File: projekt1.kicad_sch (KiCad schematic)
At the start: 19 parts, among them U1 M5STAMP-S3, U3 SCD42, U4 RV-3028-C7

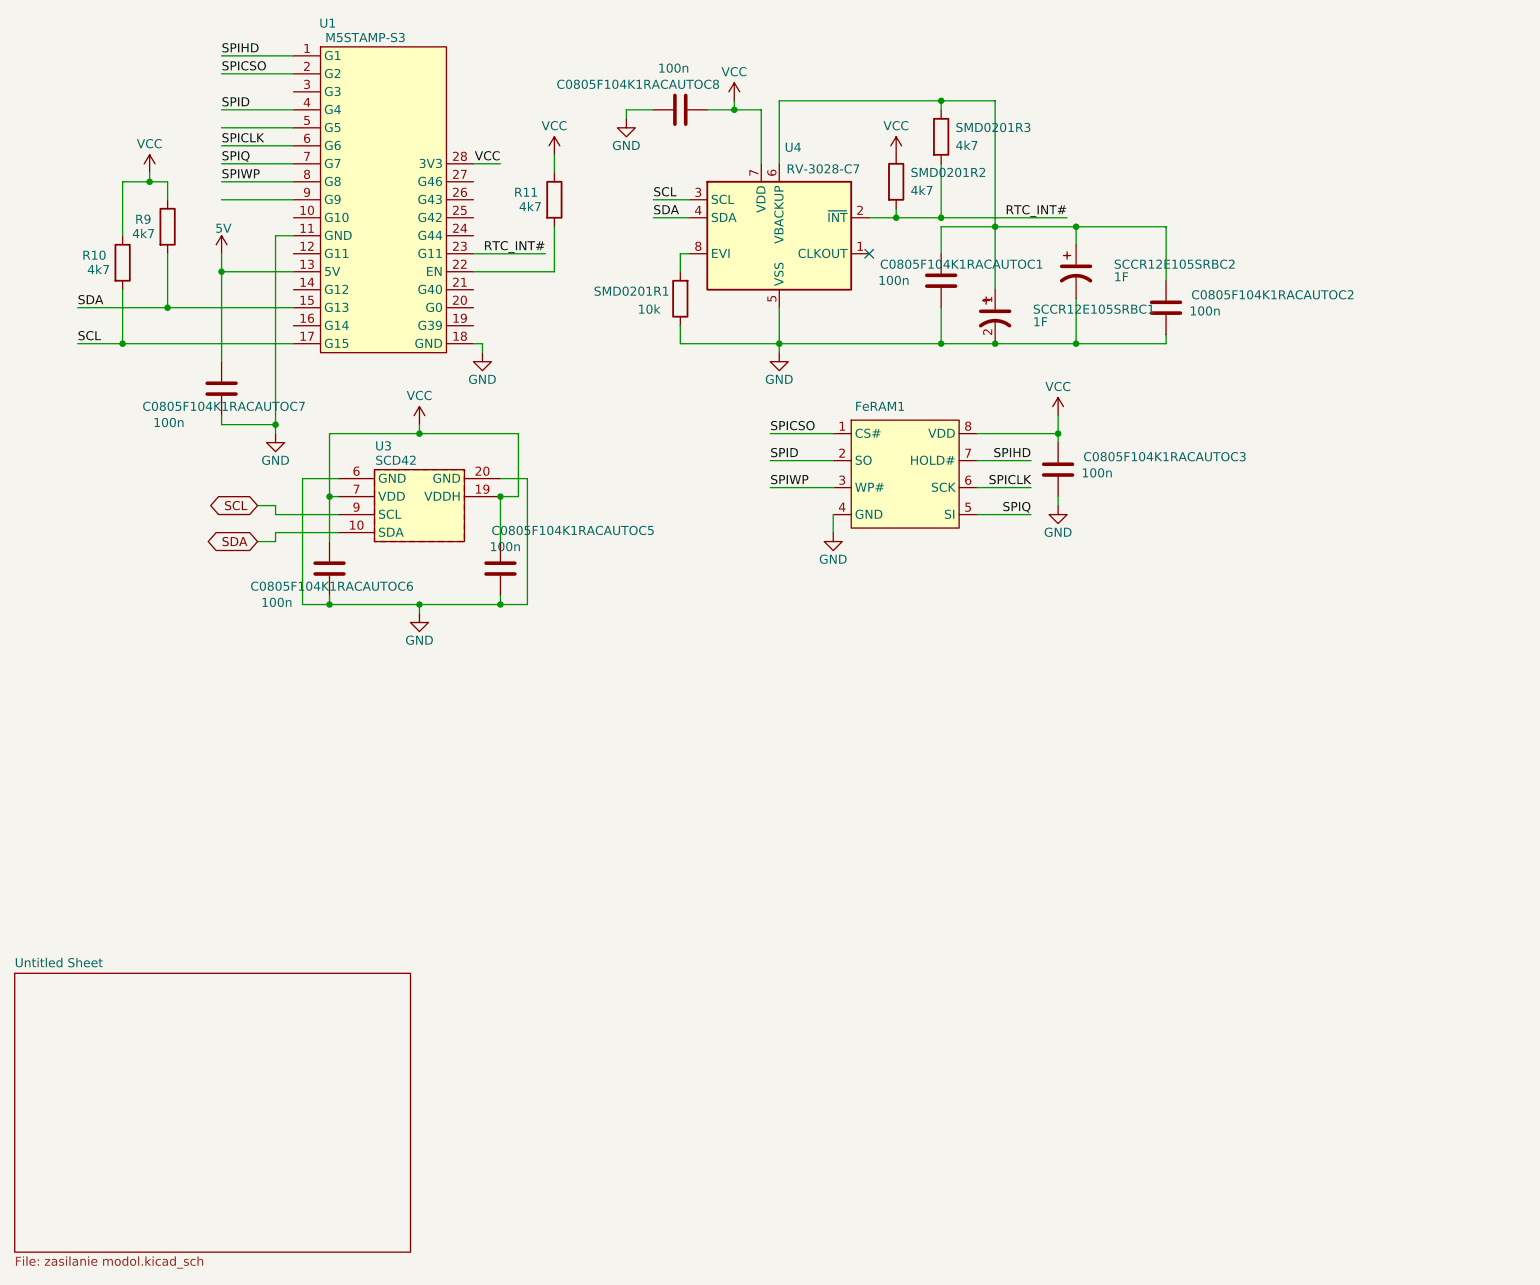
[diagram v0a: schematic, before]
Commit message: aaaaaaaaaaaaaaaaaaaaaaaaaaaaaaa
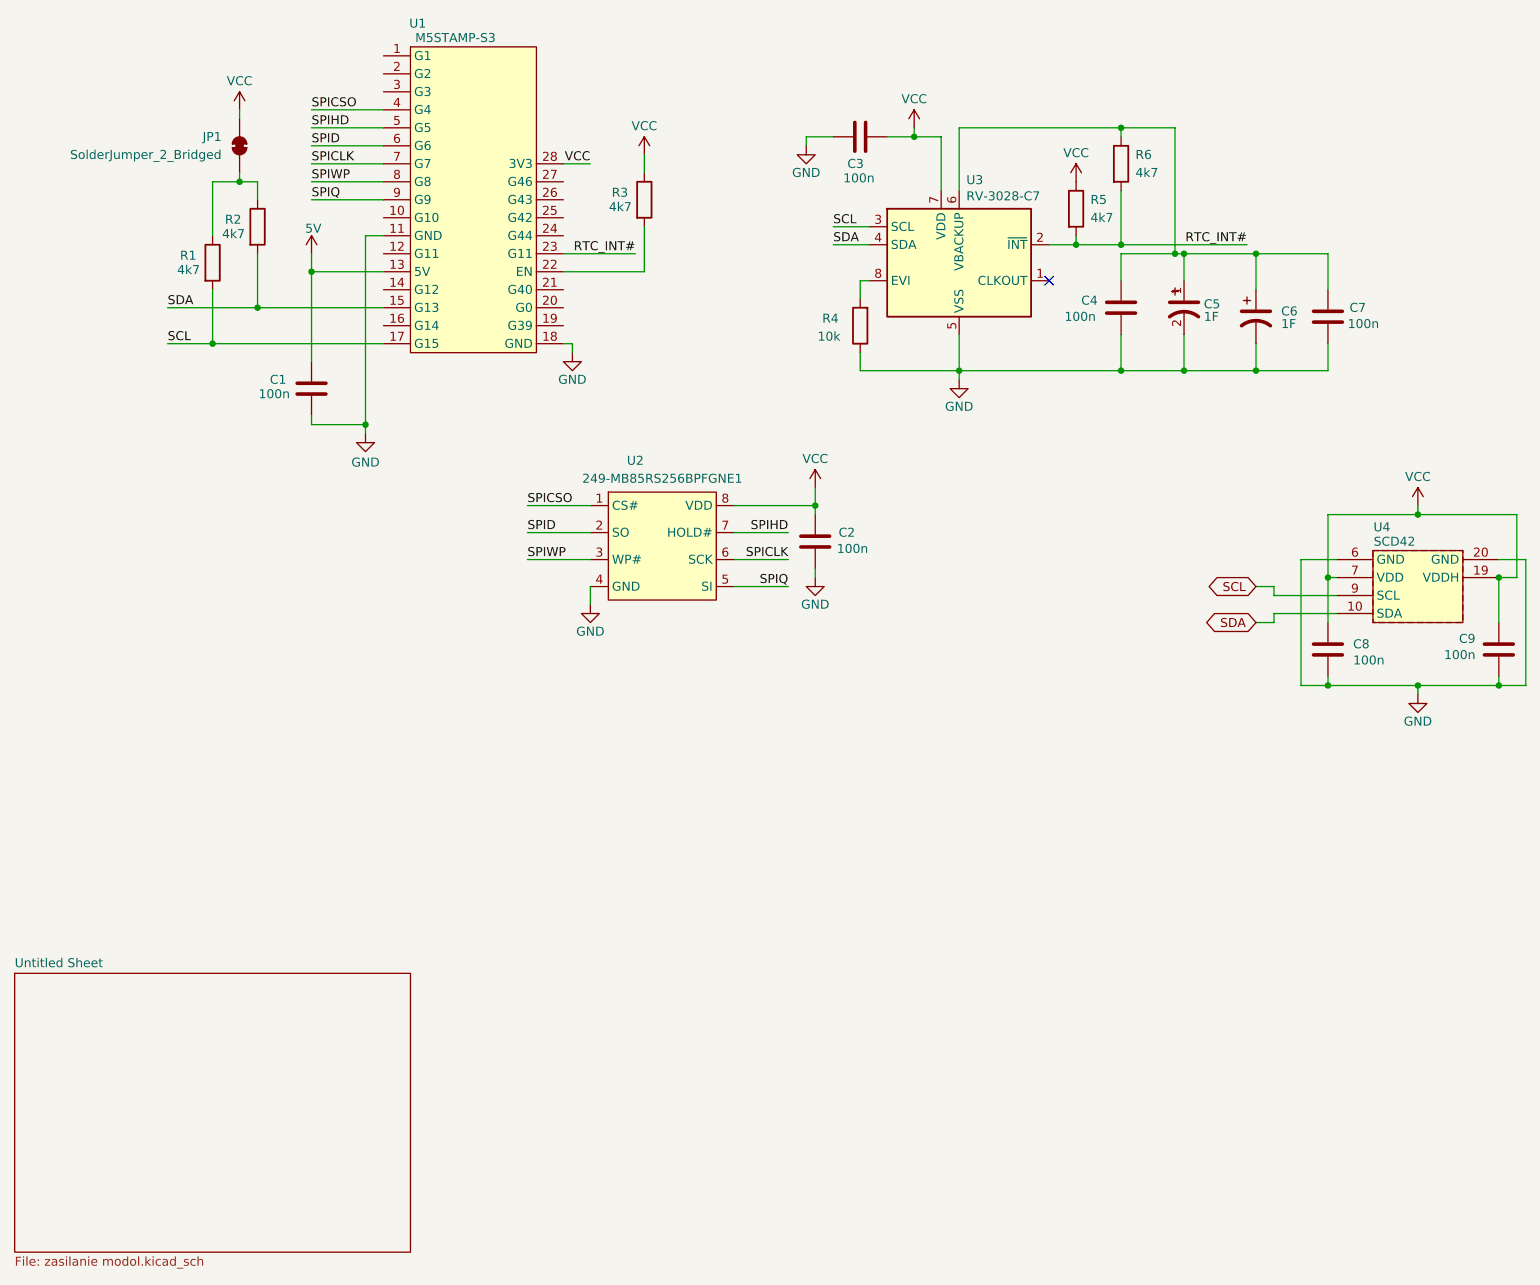
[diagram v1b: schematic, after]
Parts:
- added JP1: SolderJumper_2_Bridged, Jumper:SolderJumper-2_P1.3mm_Bridged_Pad1.0x1.5mm, symbol Jumper:SolderJumper_2_Bridged
- U2: renamed from FeRAM1; value ~ -> 249-MB85RS256BPFGNE1
- renumbered C0805F104K1RACAUTOC7 to C1, C0805F104K1RACAUTOC3 to C2, C0805F104K1RACAUTOC8 to C3, C0805F104K1RACAUTOC1 to C4, SCCR12E105SRBC1 to C5, SCCR12E105SRBC2 to C6, C0805F104K1RACAUTOC2 to C7, C0805F104K1RACAUTOC6 to C8, C0805F104K1RACAUTOC5 to C9, R10 to R1, R9 to R2, R11 to R3, SMD0201R1 to R4, SMD0201R2 to R5, SMD0201R3 to R6, U4 to U3, U3 to U4
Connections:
- net SPICLK: now also U1.7 (G7); no longer U1.6 (G6)
- net SPICSO: now also U1.4 (G4); no longer U1.2 (G2)
- net SPID: now also U1.6 (G6); no longer U1.4 (G4)
- net SPIHD: now also U1.5 (G5); no longer U1.1 (G1)
- net SPIQ: now also U1.9 (G9); no longer U1.7 (G7)
- net VCC: now also JP1.2 (B); no longer R1.1, R2.1
- new net: JP1.1 (A), R1.1, R2.1
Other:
- moved on the sheet: C1, C2, C3, C4, C5, C6, C7, C8, C9, R1, R2, R3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
